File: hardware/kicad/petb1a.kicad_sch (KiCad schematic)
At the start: 31 parts, among them J1 Socket, J2 USB_C_Receptacle_USB2.0, J3 Socket, SW1 B3U-1000P, SW2 B3U-1000P, U1 ESP32-S3-WROOM-1, U3 XC6220B331MR, U4 USBLC6-2P6

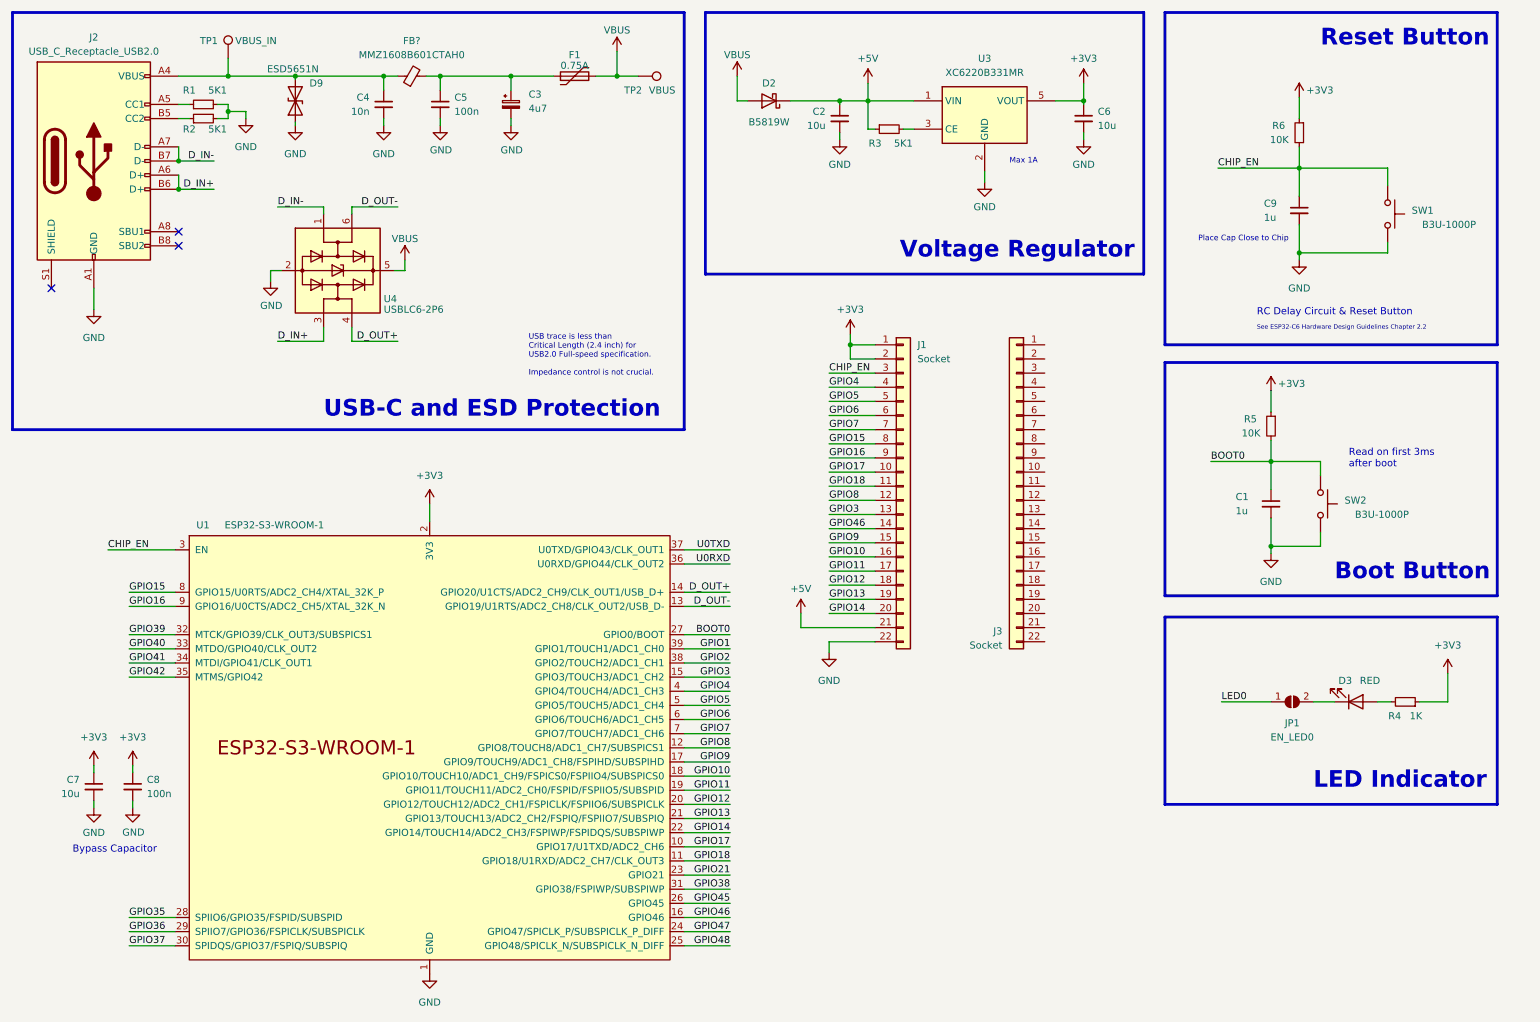
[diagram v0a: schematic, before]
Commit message: update schematics
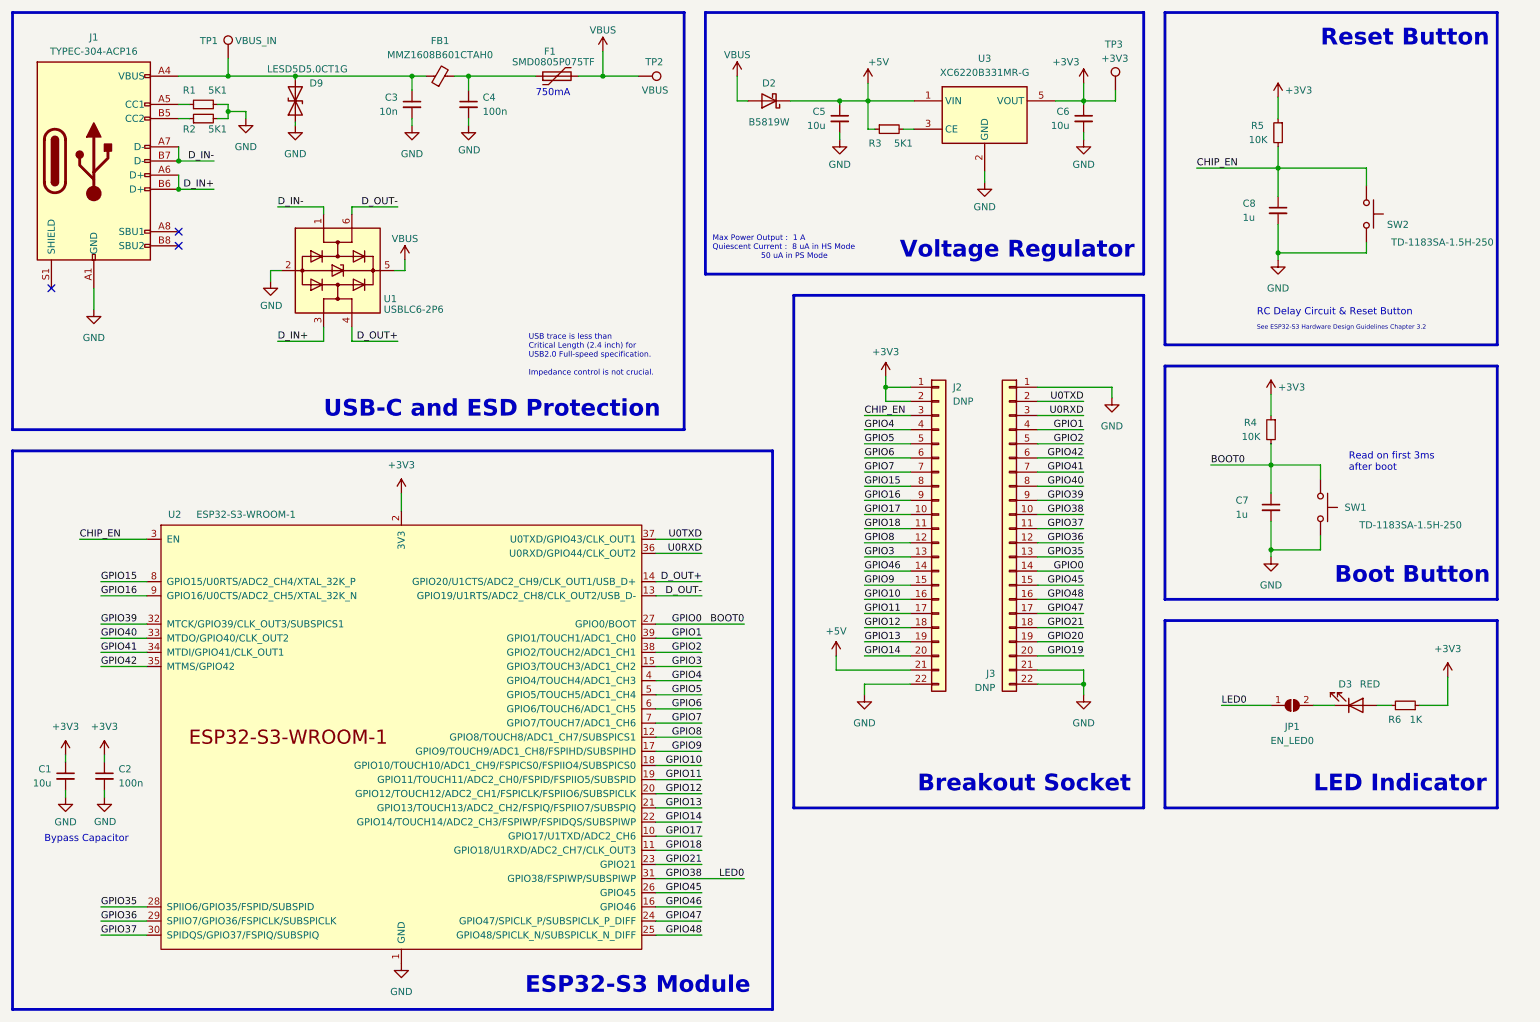
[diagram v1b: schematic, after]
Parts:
- removed C3: 4u7, symbol Device:C_Polarized_Small
- removed SW2: B3U-1000P, Button_Switch_SMD:SW_SPST_B3U-1000P, symbol Switch:SW_Push
- added SW1: TD-1183SA-1.5H-250, petb1a:KEY-SMD_L3.0-W2.5-LS4.0, symbol Switch:SW_Push
- added TP3: +3V3, TestPoint:TestPoint_Pad_D1.0mm, symbol Connector:TestPoint
- C3: renamed from C4; footprint (none) -> Capacitor_SMD:C_0603_1608Metric; Distributor (none) -> LCSC; Distributor Link (none) -> https://www.lcsc.com/product-detail/Multilayer-Ceramic-Capa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; Distributor Part Number (none) -> C100042; Manufacturer (none) -> YAGEO; Manufacturer Part Number (none) -> CC0603KRX7R9BB103; Part Description Ceramic Capacitors 16V 10nF X7R ±10% -> Ceramic Capacitors 50V 10nF X7R ±10%
- C4: renamed from C5; footprint (none) -> Capacitor_SMD:C_0603_1608Metric; Distributor (none) -> LCSC; Distributor Link (none) -> https://www.lcsc.com/product-detail/Multilayer-Ceramic-Capa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; Distributor Part Number (none) -> C1591; Manufacturer (none) -> Samsung Electro-Mechanics; Manufacturer Part Number (none) -> CL10B104KB8NNNC; Part Description Ceramic Capacitor 16V 100nF X7R ±10% -> Ceramic Capacitor 50V 100nF X7R ±10%
- C5: renamed from C2; footprint (none) -> Capacitor_SMD:C_0603_1608Metric; Distributor (none) -> LCSC; Distributor Link (none) -> https://www.lcsc.com/product-detail/Multilayer-Ceramic-Capa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; Distributor Part Number (none) -> C19702; Manufacturer (none) -> Samsung Electro-Mechanics; Manufacturer Part Number (none) -> CL10A106KP8NNNC; Part Description Ceramic Capacitor 16V 10uF X7R ±10% -> Ceramic Capacitor 10V 10uF X5R ±10%
- C6: footprint (none) -> Capacitor_SMD:C_0603_1608Metric; Distributor (none) -> LCSC; Distributor Link (none) -> https://www.lcsc.com/product-detail/Multilayer-Ceramic-Capa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; Distributor Part Number (none) -> C19702; Manufacturer (none) -> Samsung Electro-Mechanics; Manufacturer Part Number (none) -> CL10A106KP8NNNC; Part Description Ceramic Capacitor 16V 10uF X7R ±10% -> Ceramic Capacitor 10V 10uF X5R ±10%
- D2: Distributor (none) -> LCSC; Distributor Link (none) -> https://www.lcsc.com/product-detail/Schottky-Barrier-Diodes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; Distributor Part Number (none) -> C64885; Manufacturer (none) -> MDD（Microdiode Electronics); Manufacturer Part Number (none) -> B5819W; Part Description 0.05mA@40V 0.58V@1A -> SBD 40V 600mV@1A
- D9: value ESD5651N -> LESD5D5.0CT1G; footprint Capacitor_SMD:C_0402_1005Metric -> Diode_SMD:D_SOD-523; Distributor (none) -> LCSC; Distributor Link https://www.lcsc.com/product-detail/span-style-background-c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 -> https://www.lcsc.com/product-detail/Electrostatic-and-Surge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; Distributor Part Number (none) -> C383211; Manufacturer (none) -> LRC; Manufacturer Part Number (none) -> LESD5D5.0CT1G; Part Description (none) -> ESD 9.4A 18.6V 5.6V Bi-Directional 5V
- F1: value 0.75A -> SMD0805P075TF
- FB1: renamed from FB?; Distributor (none) -> LCSC; Distributor Link (none) -> https://www.lcsc.com/product-detail/Ferrite-Beads_TDK-MMZ16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; Distributor Part Number (none) -> C97120
- J1: renamed from J2; value USB_C_Receptacle_USB2.0 -> TYPEC-304-ACP16; footprint Connector_USB:USB_C_Receptacle_XKB_U262-16XN-4BVC11 -> petb1a:USB-C-SMD_TYPE-C-16P-1; Distributor (none) -> LCSC; Distributor Link (none) -> https://www.lcsc.com/product-detail/USB-Connectors_XUNPU-TY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; Distributor Part Number (none) -> C2982555; Manufacturer (none) -> XUNPU; Manufacturer Part Number (none) -> TYPEC-304-ACP16; Part Description (none) -> Type-C SMD 3A 1 Surface Mount，Right Angle 16P Female
- J2: renamed from J1; value Socket -> DNP; footprint (none) -> Connector_PinSocket_2.54mm:PinSocket_1x22_P2.54mm_Vertical; Part Description (none) -> Pin Header 1x22 P2.54mm Vertical
- J3: value Socket -> DNP; footprint (none) -> Connector_PinSocket_2.54mm:PinSocket_1x22_P2.54mm_Vertical; Part Description (none) -> Pin Header 1x22 P2.54mm Vertical
- JP1: footprint (none) -> Jumper:SolderJumper-2_P1.3mm_Open_RoundedPad1.0x1.5mm
- SW2: renamed from SW1; value B3U-1000P -> TD-1183SA-1.5H-250; footprint Button_Switch_SMD:SW_SPST_B3U-1000P -> petb1a:KEY-SMD_L3.0-W2.5-LS4.0; Distributor (none) -> LCSC; Distributor Link (none) -> https://www.lcsc.com/product-detail/Tactile-Switches_DEALON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; Distributor Part Number (none) -> C2905189; Manufacturer (none) -> DEALON; Manufacturer Part Number (none) -> TD-1183SA-1.5H-250; Part Description (none) -> Tactile Switches 2.5mm 1.5mm 3mm SMD,2.5x3mm
- U3: value XC6220B331MR -> XC6220B331MR-G; Distributor (none) -> LCSC; Distributor Link (none) -> https://www.lcsc.com/product-detail/Linear-Voltage-Regulato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; Distributor Part Number (none) -> C86534; Manufacturer (none) -> Torex Semicon; Manufacturer Part Number (none) -> XC6220B331MR-G; Part Description (none) -> LDO 50dB@(1kHz) 1A Fixed 3.3V Positive
- renumbered C7 to C1, C8 to C2, C1 to C7, C9 to C8, R5 to R4, R6 to R5, R4 to R6, U4 to U1, U1 to U2
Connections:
- net LED0 is gone; now on net GPIO38: JP1.1 (A)
- net +3V3: now also TP3.1
- net BOOT0: now also J3.14 (Pin_14), SW1.2
- net GND: now also J3.1 (Pin_1), J3.21 (Pin_21), J3.22 (Pin_22), SW1.1
- net GPIO1: now also J3.4 (Pin_4)
- net GPIO2: now also J3.5 (Pin_5)
- net GPIO21: now also J3.18 (Pin_18)
- net GPIO35: now also J3.13 (Pin_13)
- net GPIO36: now also J3.12 (Pin_12)
- net GPIO37: now also J3.11 (Pin_11)
- net GPIO38: now also J3.10 (Pin_10)
- net GPIO39: now also J3.9 (Pin_9)
- net GPIO40: now also J3.8 (Pin_8)
- net GPIO41: now also J3.7 (Pin_7)
- net GPIO42: now also J3.6 (Pin_6)
- net GPIO45: now also J3.15 (Pin_15)
- net GPIO47: now also J3.17 (Pin_17)
- net GPIO48: now also J3.16 (Pin_16)
- net U0RXD: now also J3.3 (Pin_3)
- net U0TXD: now also J3.2 (Pin_2)
- net GPIO20: now reaches J3.19 (Pin_19)
- net GPIO19: now reaches J3.20 (Pin_20)
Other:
- note added: "750mA"
- note added: "Breakout Socket"
- note added: "ESP32-S3 Module"
- note added: "Max Power Output : 1 A Quiescent Current : 8 uA in HS Mode 50 uA in PS Mode"
- note added: "See ESP32-S3 Hardware Design Guidelines Chapter 3.2"
- note removed: "Max 1A"
- note removed: "Place Cap Close to Chip"
- note removed: "See ESP32-C6 Hardware Design Guidelines Chapter 2.2"
- title: PETB1A -> Teapotlabs PETB1A
- moved on the sheet: C1, C2, C3, C4, C7, C8, D3, F1, FB1, J2, J3, JP1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
